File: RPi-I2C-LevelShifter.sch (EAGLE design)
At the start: 8 parts, among them Q1 2N7002, Q2 2N7002

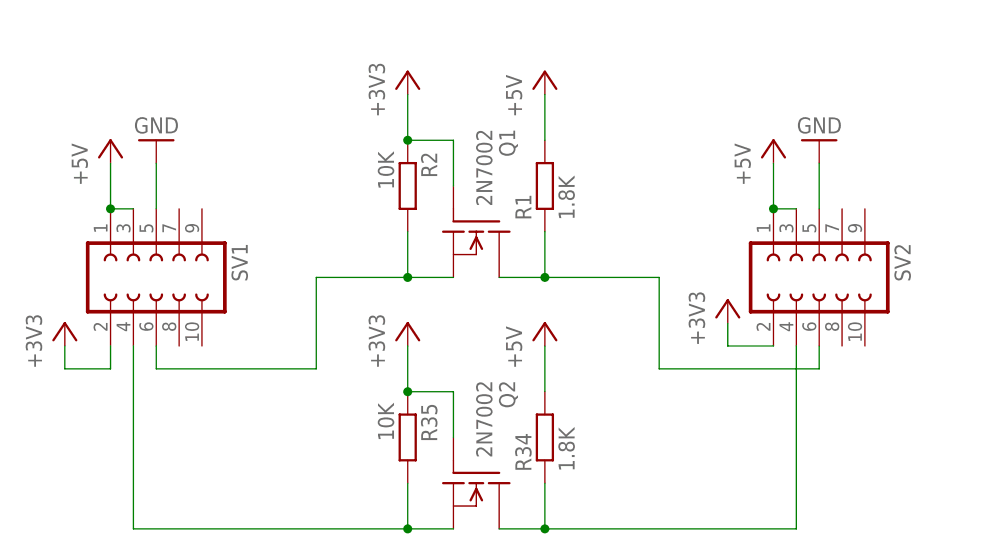
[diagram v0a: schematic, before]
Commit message: fixed error
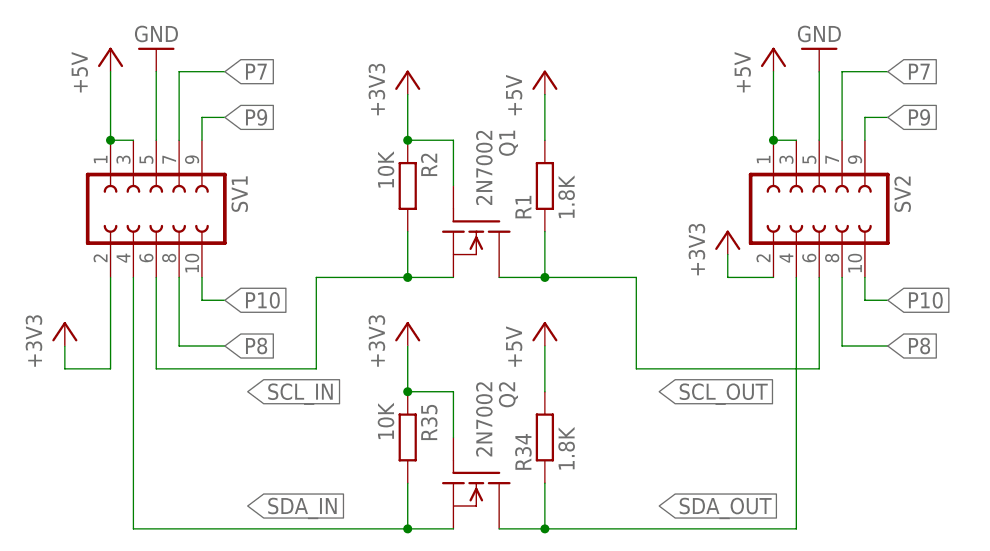
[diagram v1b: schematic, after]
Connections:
- new net P10: SV1.10, SV2.10
- new net P7: SV1.7, SV2.7
- new net P8: SV1.8, SV2.8
- new net P9: SV1.9, SV2.9
- new net SCL_OUT: Q1.D, R1.1, SV2.6
- new net SDA_OUT: Q2.D, R34.1, SV2.4
- net SCL_IN: now also Q1.S, R2.2, SV1.6; no longer Q2.D, Q2.S, R34.1, R35.2, SV1.4, SV2.4
- net SDA_IN: now also Q2.S, R35.2, SV1.4; no longer Q1.D, Q1.S, R1.1, R2.2, SV1.6, SV2.6
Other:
- moved on the sheet: SV1, SV2
